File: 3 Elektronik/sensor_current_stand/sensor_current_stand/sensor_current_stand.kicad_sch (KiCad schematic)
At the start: 3 parts, among them J1 Conn_01x02_Socket, J2 Conn_01x02_Socket, J7 USB_B

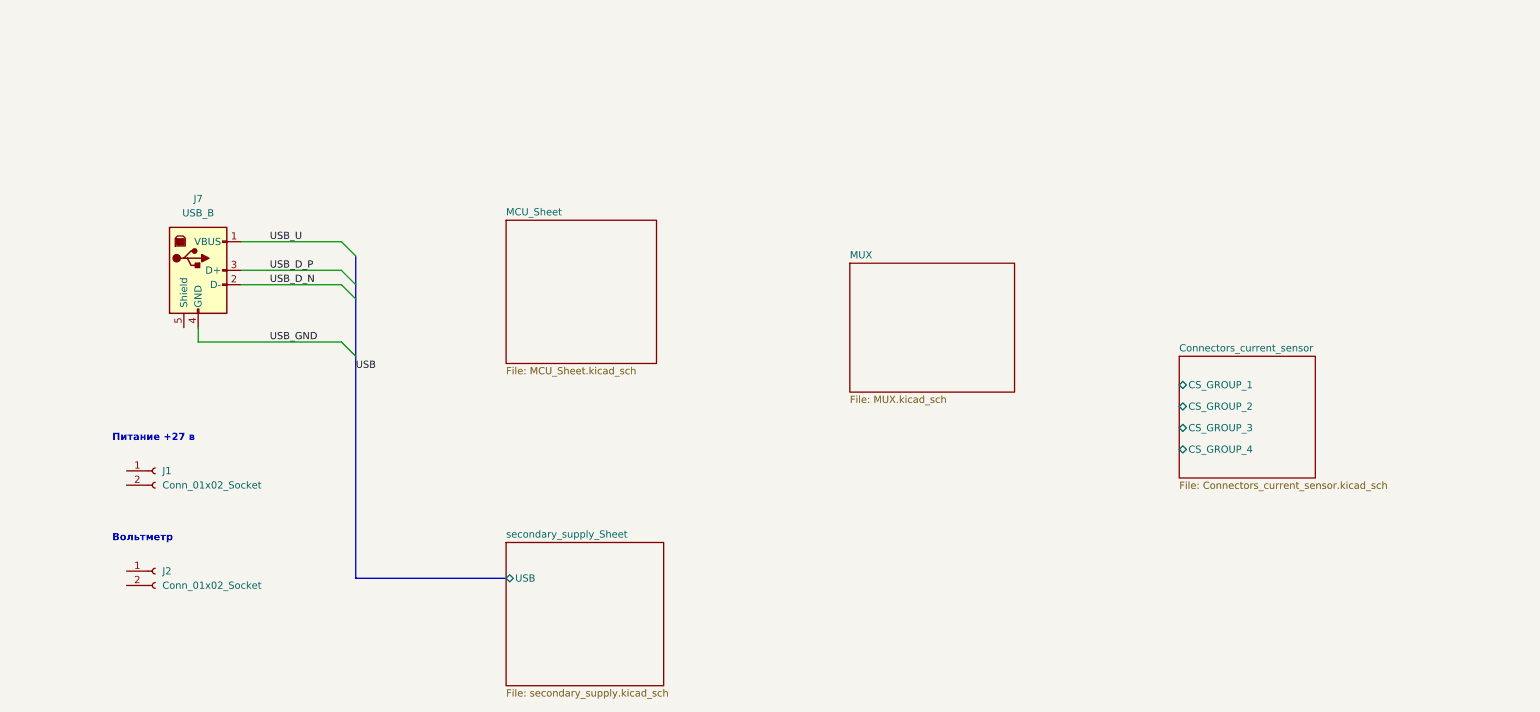
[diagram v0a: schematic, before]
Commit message: разработка
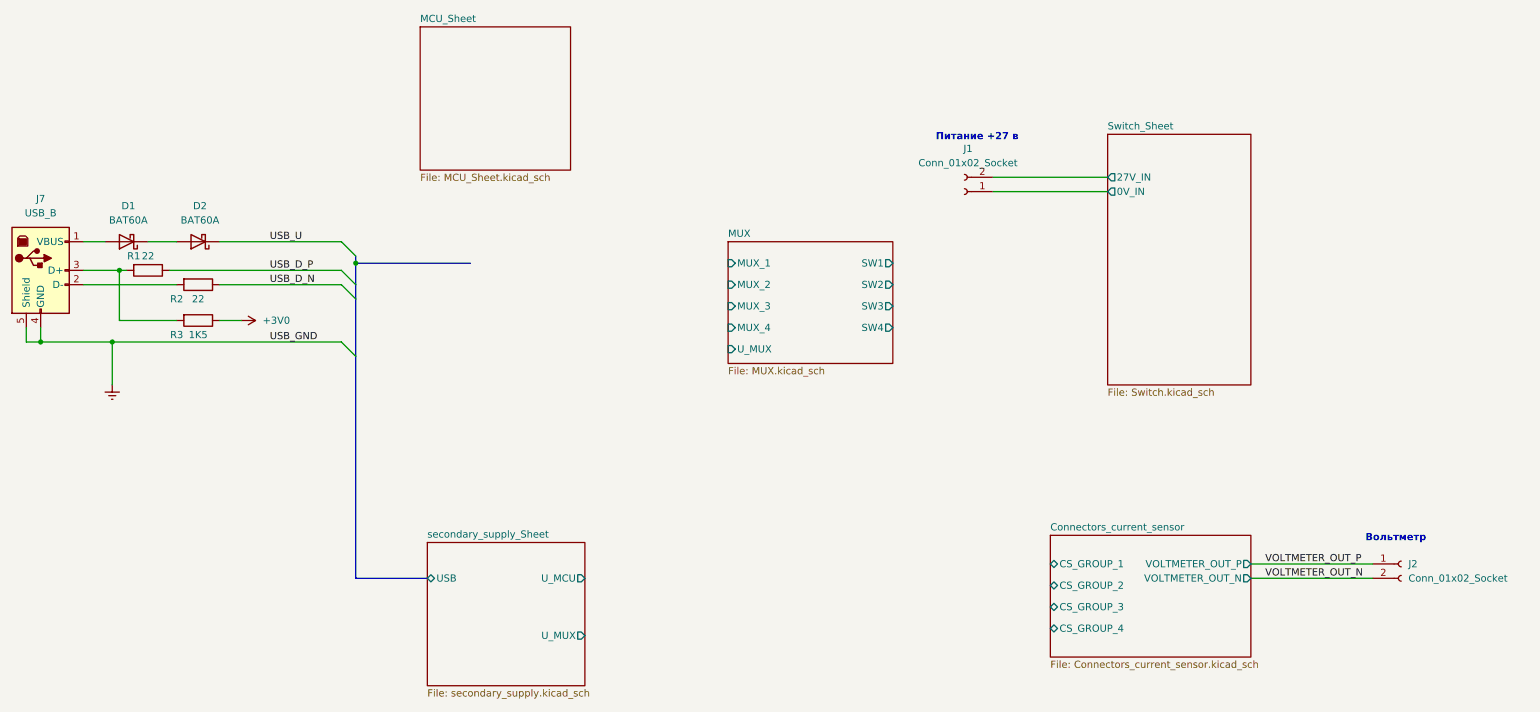
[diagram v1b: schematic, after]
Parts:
- added D1, D2: BAT60A, Diode_SMD:D_SOD-323, symbol Diode:BAT60A
- added R1, R2: 22, Resistor_SMD:R_1206_3216Metric_Pad1.30x1.75mm_HandSolder, symbol Device:R
- added R3: 1K5, Resistor_SMD:R_1206_3216Metric_Pad1.30x1.75mm_HandSolder, symbol Device:R
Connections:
- net USB_GND is gone; now on net Earth: J7.4 (GND)
- net USB_D_N: now also R2.1; no longer J7.2 (D-)
- net USB_D_P: now also R1.1; no longer J7.3 (D+)
- net USB_U: now also D2.1 (K); no longer J7.1 (VBUS)
- net Switch_Sheet/0V_IN: now reaches J1.1 (Pin_1)
- net Switch_Sheet/27V_IN: now reaches J1.2 (Pin_2)
- net VOLTMETER_OUT_P: now reaches J2.1 (Pin_1)
- net VOLTMETER_OUT_N: now reaches J2.2 (Pin_2)
- net Earth: now reaches J7.5 (Shield)
- new net: J7.2 (D-), R2.2
- new net: D1.1 (K), D2.2 (A)
- new net: D1.2 (A), J7.1 (VBUS)
- new net: J7.3 (D+), R1.2, R3.2
- new net +3V0: R3.1
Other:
- added sheet Switch_Sheet (Switch.kicad_sch)
- sheet Connectors_current_sensor ports: added VOLTMETER_OUT_N, VOLTMETER_OUT_P; removed none
- sheet MUX ports: added MUX_1, MUX_2, MUX_3, MUX_4, SW1, SW2, SW3, SW4, U_MUX; removed none
- sheet secondary_supply_Sheet ports: added U_MCU, U_MUX; removed none
- moved on the sheet: J1, J2, J7

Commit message: quarz
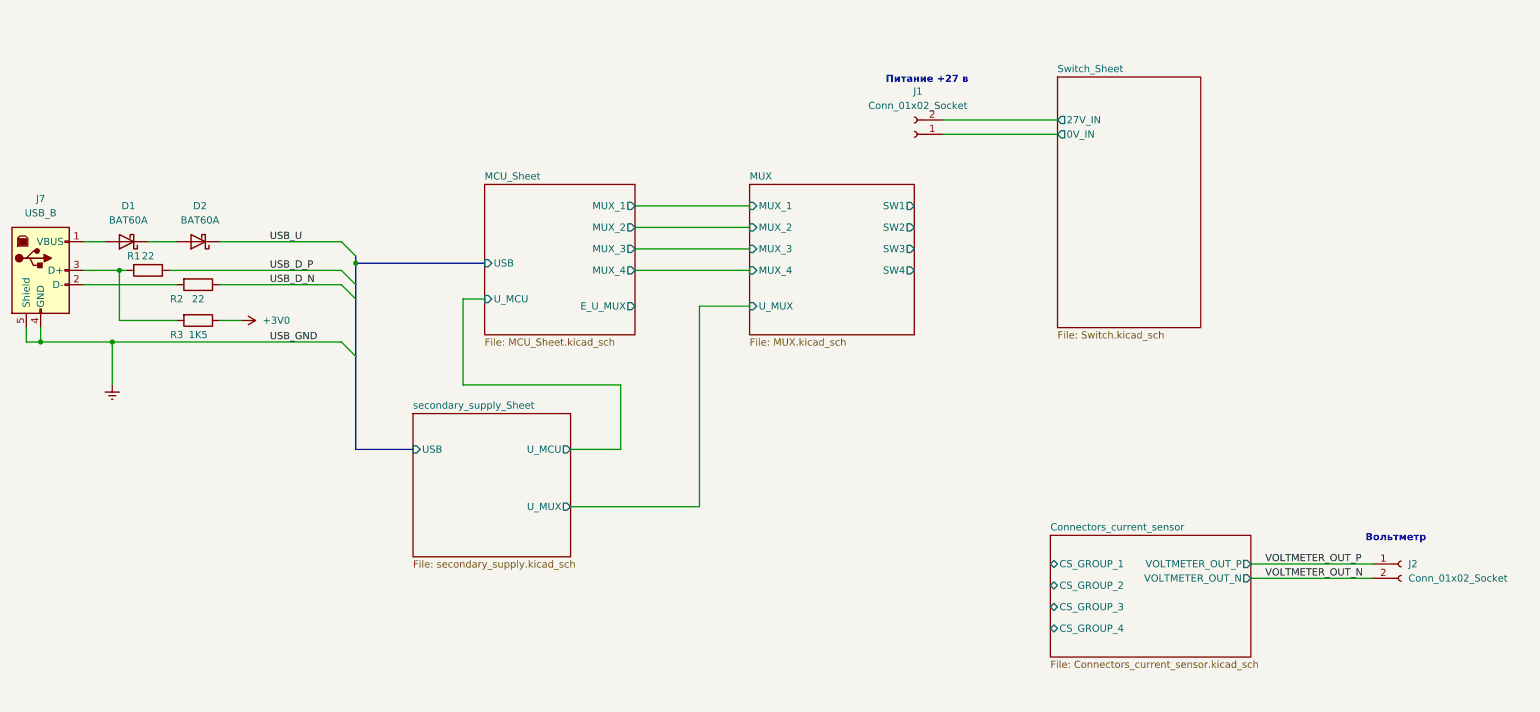
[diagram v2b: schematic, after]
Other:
- sheet MCU_Sheet ports: added E_U_MUX, MUX_1, MUX_2, MUX_3, MUX_4, USB, U_MCU; removed none
- moved on the sheet: J1
